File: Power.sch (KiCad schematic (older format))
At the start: 27 parts, among them J3 Barrel_Jack_Switch, J4 USB_B_Micro, SW1 2MS1-T1-B2-M7-S-E, U4 MCW03, U5 MCW03, U6 NJM7809, U7 NJM7909

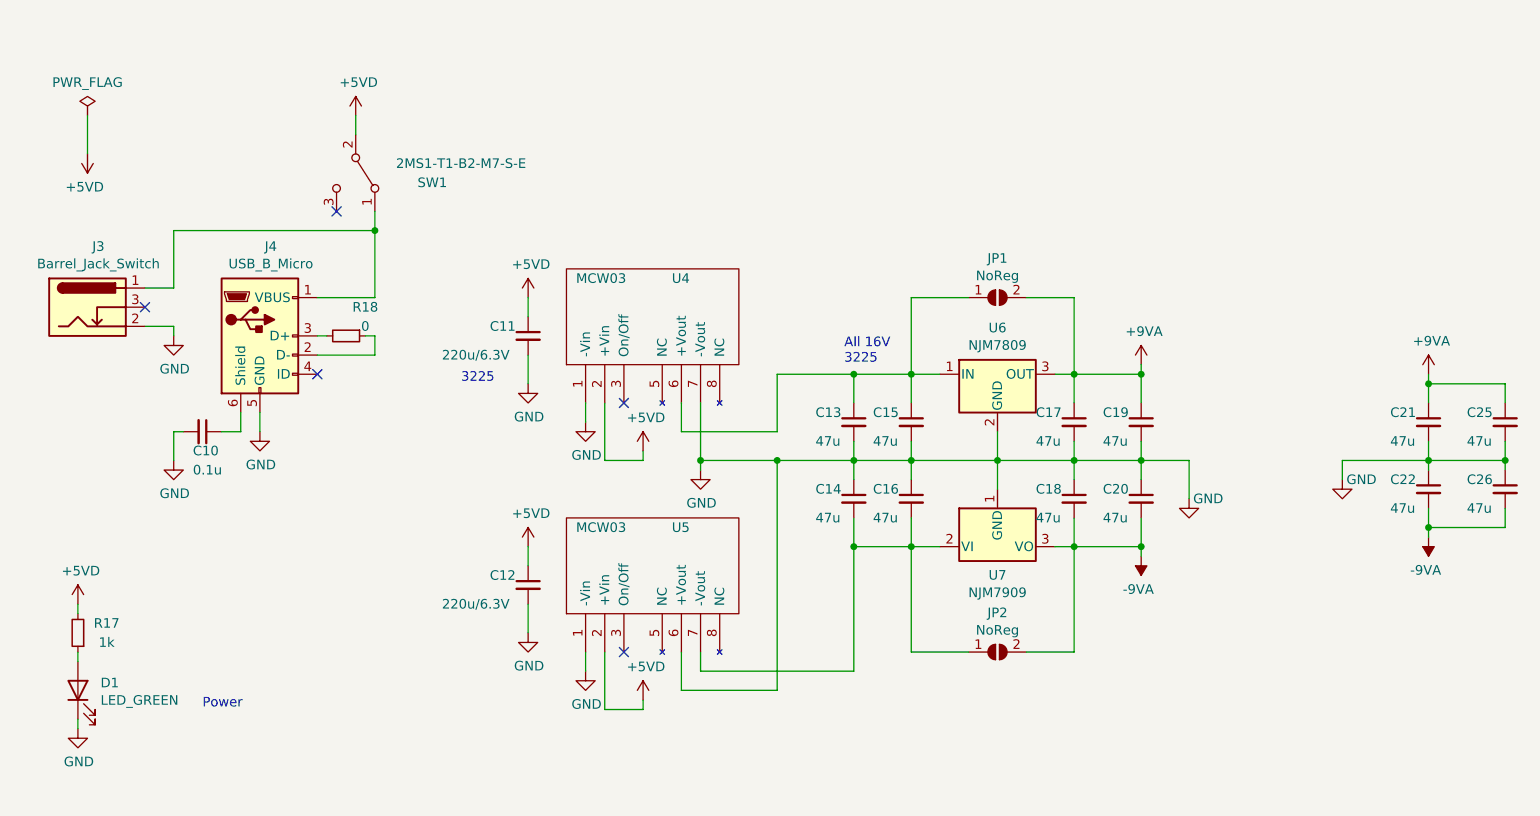
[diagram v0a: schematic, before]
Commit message: Rev.A 完成
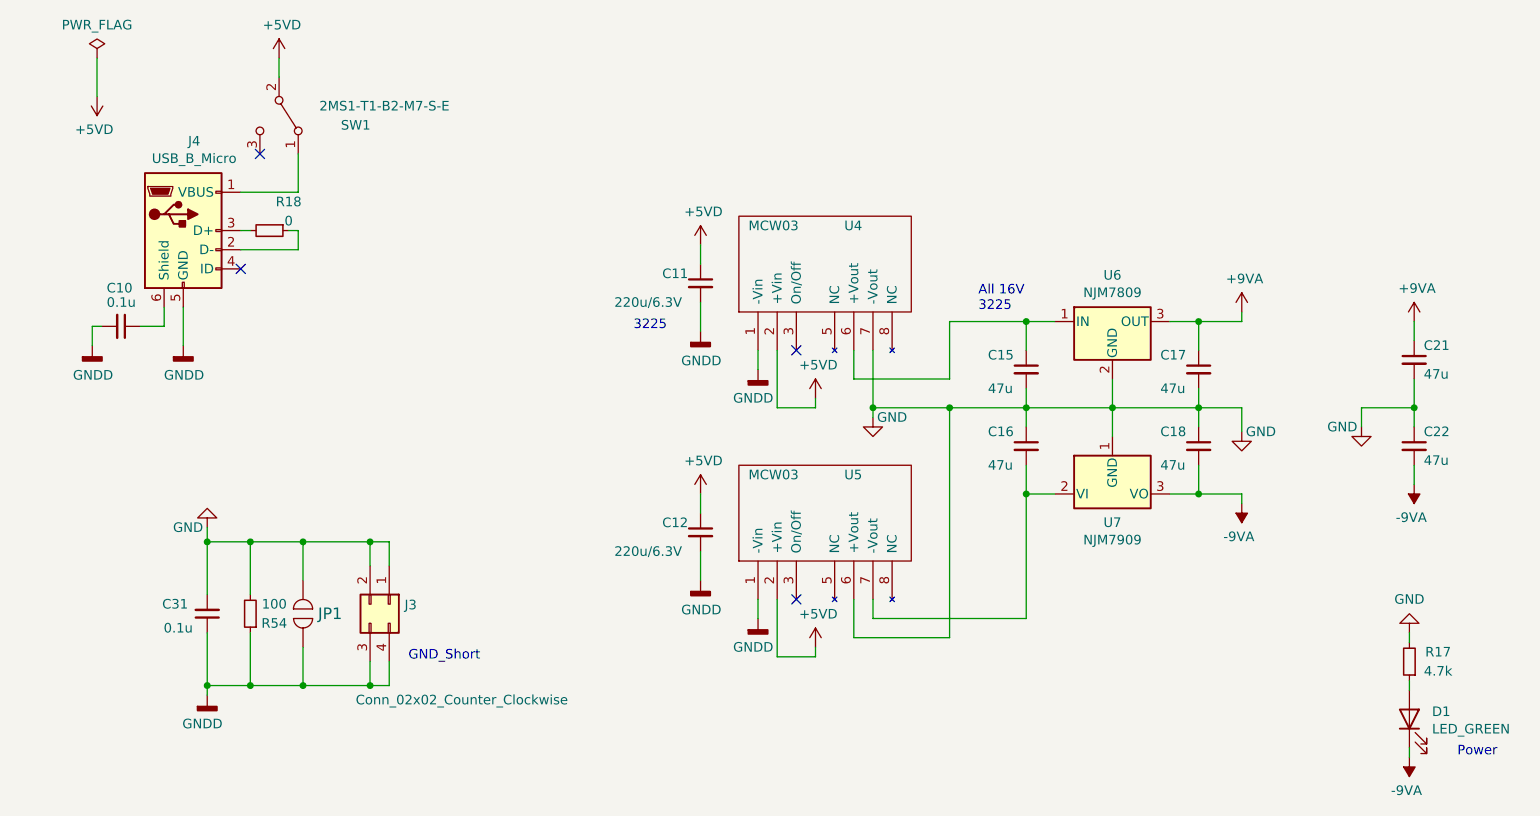
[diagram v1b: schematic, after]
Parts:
- removed C13, C14, C19, C20, C25, C26: 47u, Capacitor_SMD:C_1210_3225Metric_Pad1.42x2.65mm_HandSolder, symbol Device:C_Small
- removed J3: Barrel_Jack_Switch, hastech:MJ-179P, symbol Connector:Barrel_Jack_Switch
- removed JP1, JP2: NoReg, Jumper:SolderJumper-2_P1.3mm_Open_TrianglePad1.0x1.5mm, symbol Jumper:SolderJumper_2_Open
- added C31: 0.1u, Capacitor_SMD:C_0603_1608Metric_Pad1.05x0.95mm_HandSolder, symbol Device:C_Small
- added J3: Conn_02x02_Counter_Clockwise, Connector_PinHeader_2.54mm:PinHeader_2x02_P2.54mm_Vertical, symbol Connector_Generic:Conn_02x02_Counter_Clockwise
- added JP1: UserShort, Jumper:SolderJumper-2_P1.3mm_Open_RoundedPad1.0x1.5mm, symbol kamiya:UserShort
- added R54: 100, Resistor_SMD:R_0603_1608Metric_Pad1.05x0.95mm_HandSolder, symbol Device:R_Small
- R17: value 1k -> 4.7k
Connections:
- net +5VD: no longer R17.2
- net -9VA: now also D1.1 (K)
- net GND: now also R17.2, C31.2, J3.1 (Pin_1), J3.2 (Pin_2), JP1.1, R54.2; no longer C10.2, C11.2, C12.2, D1.1 (K), J4.5 (GND), U4.1 (-Vin), U5.1 (-Vin)
- new net GNDD: C10.2, C11.2, C12.2, C31.1, J3.3 (Pin_3), J3.4 (Pin_4), J4.5 (GND), JP1.2, R54.1, U4.1 (-Vin), U5.1 (-Vin)
- no-connect marks 5 -> 4
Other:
- note added: "GND_Short"
- moved on the sheet: C10, C11, C12, C15, C16, C17, C18, C21, C22, D1, J4, R17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
